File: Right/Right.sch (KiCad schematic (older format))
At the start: 188 parts, among them SW0 SW_PUSH, SW1 SW_PUSH, SW10 SW_PUSH, SW100 SW_PUSH, SW1000 SW_Push_Dual_R, SW1001 SW_Push_Dual_R, SW1002 SW_Push_Dual_R, SW1003 SW_Push_Dual_R, SW1004 SW_Push_Dual_R, SW1005 SW_Push_Dual_R, SW101 SW_PUSH, SW102 SW_PUSH, SW103 SW_PUSH, SW104 SW_PUSH, SW105 SW_PUSH, SW106 SW_PUSH, SW11 SW_PUSH, SW110 SW_PUSH, SW111 SW_PUSH, SW112 SW_PUSH, SW113 SW_PUSH, SW114 SW_PUSH, SW115 SW_PUSH, SW116 SW_PUSH, SW12 SW_PUSH, SW13 SW_PUSH, SW14 SW_PUSH, SW15 SW_PUSH, SW2 SW_PUSH, SW20 SW_PUSH, SW21 SW_PUSH, SW22 SW_PUSH, SW23 SW_PUSH, SW24 SW_PUSH, SW25 SW_PUSH, SW3 SW_PUSH, SW30 SW_PUSH, SW31 SW_PUSH, SW32 SW_PUSH, SW33 SW_PUSH, SW34 SW_PUSH, SW35 SW_PUSH, SW4 SW_PUSH, SW40 SW_PUSH, SW41 SW_PUSH, SW42 SW_PUSH, SW43 SW_PUSH, SW44 SW_PUSH, SW45 SW_PUSH, SW5 SW_PUSH, SW50 SW_PUSH, SW51 SW_PUSH, SW52 SW_PUSH, SW53 SW_PUSH, SW54 SW_PUSH, SW60 SW_PUSH, SW61 SW_PUSH, SW62 SW_PUSH, SW63 SW_PUSH, SW64 SW_PUSH, SW65 SW_PUSH, SW66 SW_PUSH, SW70 SW_PUSH, SW71 SW_PUSH, SW72 SW_PUSH, SW73 SW_PUSH, SW74 SW_PUSH, SW75 SW_PUSH, SW76 SW_PUSH, SW77 SW_PUSH, SW80 SW_PUSH, SW81 SW_PUSH, SW82 SW_PUSH, SW83 SW_PUSH, SW84 SW_PUSH, SW85 SW_PUSH, SW86 SW_PUSH, SW87 SW_PUSH, SW90 SW_PUSH, SW91 SW_PUSH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

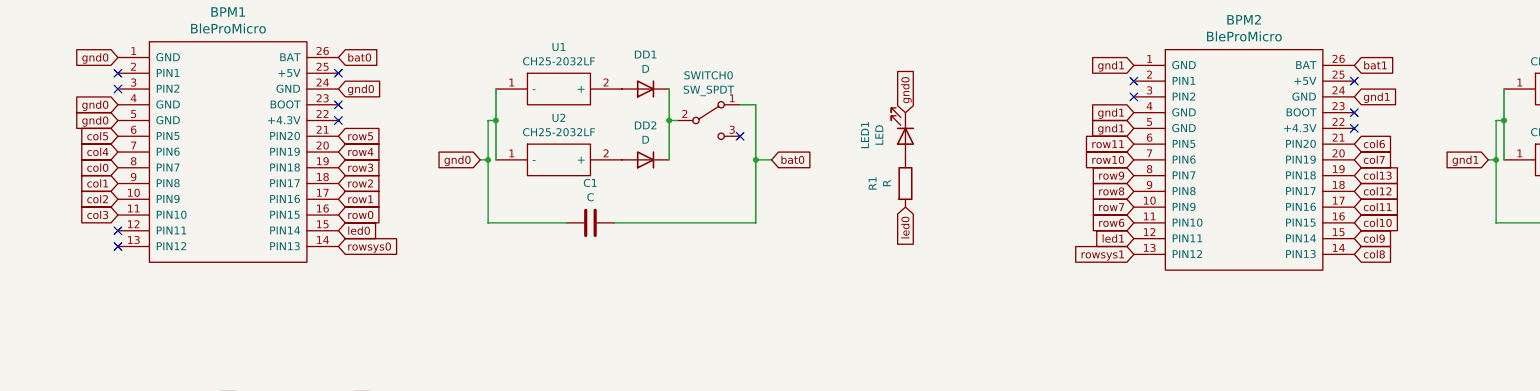
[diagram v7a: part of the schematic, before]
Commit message: 完成
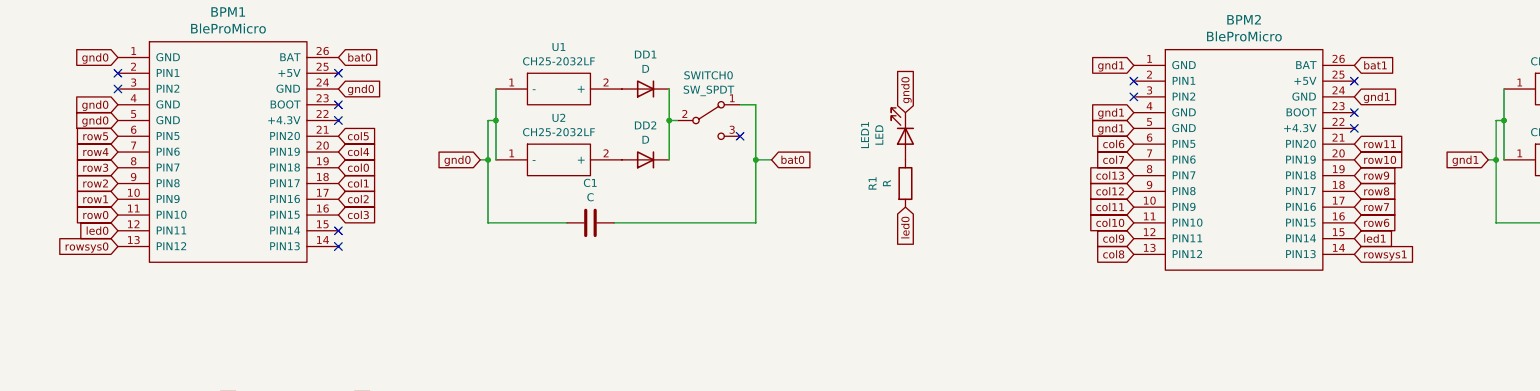
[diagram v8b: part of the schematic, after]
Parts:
- BPM1, BPM2: footprint mylibrary:BLEMicroPro -> mylibrary:BLEMicroPro_reversed
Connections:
- net col0: now also BPM1.19 (PIN18); no longer BPM1.8 (PIN7)
- net col1: now also BPM1.18 (PIN17); no longer BPM1.9 (PIN8)
- net col10: now also BPM2.11 (PIN10); no longer BPM2.16 (PIN15)
- net col11: now also BPM2.10 (PIN9); no longer BPM2.17 (PIN16)
- net col12: now also BPM2.9 (PIN8); no longer BPM2.18 (PIN17)
- net col13: now also BPM2.8 (PIN7); no longer BPM2.19 (PIN18)
- net col2: now also BPM1.17 (PIN16); no longer BPM1.10 (PIN9)
- net col3: now also BPM1.16 (PIN15); no longer BPM1.11 (PIN10)
- net col4: now also BPM1.20 (PIN19); no longer BPM1.7 (PIN6)
- net col5: now also BPM1.21 (PIN20); no longer BPM1.6 (PIN5)
- net col6: now also BPM2.6 (PIN5); no longer BPM2.21 (PIN20)
- net col7: now also BPM2.7 (PIN6); no longer BPM2.20 (PIN19)
- net col8: now also BPM2.13 (PIN12); no longer BPM2.14 (PIN13)
- net col9: now also BPM2.12 (PIN11); no longer BPM2.15 (PIN14)
- net led0: now also BPM1.12 (PIN11); no longer BPM1.15 (PIN14)
- net led1: now also BPM2.15 (PIN14); no longer BPM2.12 (PIN11)
- net row0: now also BPM1.11 (PIN10); no longer BPM1.16 (PIN15)
- net row1: now also BPM1.10 (PIN9); no longer BPM1.17 (PIN16)
- net row10: now also BPM2.20 (PIN19); no longer BPM2.7 (PIN6)
- net row11: now also BPM2.21 (PIN20); no longer BPM2.6 (PIN5)
- net row2: now also BPM1.9 (PIN8); no longer BPM1.18 (PIN17)
- net row3: now also BPM1.8 (PIN7); no longer BPM1.19 (PIN18)
- net row4: now also BPM1.7 (PIN6); no longer BPM1.20 (PIN19)
- net row5: now also BPM1.6 (PIN5); no longer BPM1.21 (PIN20)
- net row6: now also BPM2.16 (PIN15); no longer BPM2.11 (PIN10)
- net row7: now also BPM2.17 (PIN16); no longer BPM2.10 (PIN9)
- net row8: now also BPM2.18 (PIN17); no longer BPM2.9 (PIN8)
- net row9: now also BPM2.19 (PIN18); no longer BPM2.8 (PIN7)
- net rowsys0: now also BPM1.13 (PIN12); no longer BPM1.14 (PIN13)
- net rowsys1: now also BPM2.14 (PIN13); no longer BPM2.13 (PIN12)
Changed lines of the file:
@@
 F 0 "BPM1" H 2800 3837 60  0000 C CNN
 F 1 "BleProMicro" H 2800 3731 60  0000 C CNN
-F 2 "mylibrary:BLEMicroPro" H 2900 1650 60  0001 C CNN
+F 2 "mylibrary:BLEMicroPro_reversed" H 2900 1650 60  0001 C CNN
 F 3 "" H 2900 1650 60  0000 C CNN
 	1    2800 2700
@@
 Text GLabel 7100 2800 3    50   Input ~ 0
 led0
-Text GLabel 3500 2950 2    50   Input ~ 0
+Text GLabel 2100 2950 0    50   Input ~ 0
 led0
 NoConn ~ 2100 2050
@@
 	4450 2500 4450 2250
 NoConn ~ 6050 2350
-Text GLabel 3500 3050 2    50   Input ~ 0
+Text GLabel 2100 3050 0    50   Input ~ 0
 rowsys0
 $Comp
@@
 F 0 "BPM2" H 9250 3887 60  0000 C CNN
 F 1 "BleProMicro" H 9250 3781 60  0000 C CNN
-F 2 "mylibrary:BLEMicroPro" H 9350 1700 60  0001 C CNN
+F 2 "mylibrary:BLEMicroPro_reversed" H 9350 1700 60  0001 C CNN
 F 3 "" H 9350 1700 60  0000 C CNN
 	1    9250 2750
@@
 Wire Wire Line
 	4250 9250 5950 9250
-NoConn ~ 2100 3050
-NoConn ~ 2100 2950
+Text GLabel 3500 2350 2    50   Input ~ 0
+col5
+Text GLabel 3500 2450 2    50   Input ~ 0
+col4
+Text GLabel 3500 2850 2    50   Input ~ 0
+col3
+Text GLabel 3500 2750 2    50   Input ~ 0
+col2
+Text GLabel 3500 2650 2    50   Input ~ 0
+col1
+Text GLabel 3500 2550 2    50   Input ~ 0
+col0
+Text GLabel 2100 2850 0    50   Input ~ 0
+row0
+Text GLabel 2100 2750 0    50   Input ~ 0
+row1
+Text GLabel 2100 2650 0    50   Input ~ 0
+row2
+Text GLabel 2100 2550 0    50   Input ~ 0
+row3
+Text GLabel 2100 2450 0    50   Input ~ 0
+row4
 Text GLabel 2100 2350 0    50   Input ~ 0
-col5
-Text GLabel 2100 2450 0    50   Input ~ 0
-col4
-Text GLabel 2100 2850 0    50   Input ~ 0
-col3
-Text GLabel 2100 2750 0    50   Input ~ 0
-col2
-Text GLabel 2100 2650 0    50   Input ~ 0
-col1
-Text GLabel 2100 2550 0    50   Input ~ 0
-col0
-Text GLabel 3500 2850 2    50   Input ~ 0
-row0
-Text GLabel 3500 2750 2    50   Input ~ 0
-row1
-Text GLabel 3500 2650 2    50   Input ~ 0
-row2
-Text GLabel 3500 2550 2    50   Input ~ 0
-row3
-Text GLabel 3500 2450 2    50   Input ~ 0
-row4
-Text GLabel 3500 2350 2    50   Input ~ 0
 row5
+Text GLabel 9950 3000 2    50   Input ~ 0
+led1
+Text GLabel 9950 3100 2    50   Input ~ 0
+rowsys1
+Text GLabel 9950 2400 2    50   Input ~ 0
+row11
+Text GLabel 9950 2500 2    50   Input ~ 0
+row10
+Text GLabel 9950 2600 2    50   Input ~ 0
+row9
+Text GLabel 9950 2700 2    50   Input ~ 0
+row8
+Text GLabel 9950 2800 2    50   Input ~ 0
+row7
+Text GLabel 9950 2900 2    50   Input ~ 0
+row6
+Text GLabel 8550 2400 0    50   Input ~ 0
+col6
+Text GLabel 8550 2500 0    50   Input ~ 0
+col7
+Text GLabel 8550 3100 0    50   Input ~ 0
+col8
 Text GLabel 8550 3000 0    50   Input ~ 0
-led1
-Text GLabel 8550 3100 0    50   Input ~ 0
-rowsys1
-Text GLabel 8550 2400 0    50   Input ~ 0
-row11
-Text GLabel 8550 2500 0    50   Input ~ 0
-row10
+col9
+Text GLabel 8550 2900 0    50   Input ~ 0
+col10
+Text GLabel 8550 2800 0    50   Input ~ 0
+col11
+Text GLabel 8550 2700 0    50   Input ~ 0
+col12
 Text GLabel 8550 2600 0    50   Input ~ 0
-row9
-Text GLabel 8550 2700 0    50   Input ~ 0
-row8
-Text GLabel 8550 2800 0    50   Input ~ 0
-row7
-Text GLabel 8550 2900 0    50   Input ~ 0
-row6
-Text GLabel 9950 2400 2    50   Input ~ 0
-col6
-Text GLabel 9950 2500 2    50   Input ~ 0
-col7
-Text GLabel 9950 3100 2    50   Input ~ 0
-col8
-Text GLabel 9950 3000 2    50   Input ~ 0
-col9
-Text GLabel 9950 2900 2    50   Input ~ 0
-col10
-Text GLabel 9950 2800 2    50   Input ~ 0
-col11
-Text GLabel 9950 2700 2    50   Input ~ 0
-col12
-Text GLabel 9950 2600 2    50   Input ~ 0
 col13
+NoConn ~ 3500 2950
+NoConn ~ 3500 3050
 $EndSCHEMATC
